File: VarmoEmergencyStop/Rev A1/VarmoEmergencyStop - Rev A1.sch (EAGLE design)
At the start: 6 parts, among them J1 22-05-7028-02, X1 NC3MAV, X2 NC3FAV2, X3 NC3MAV

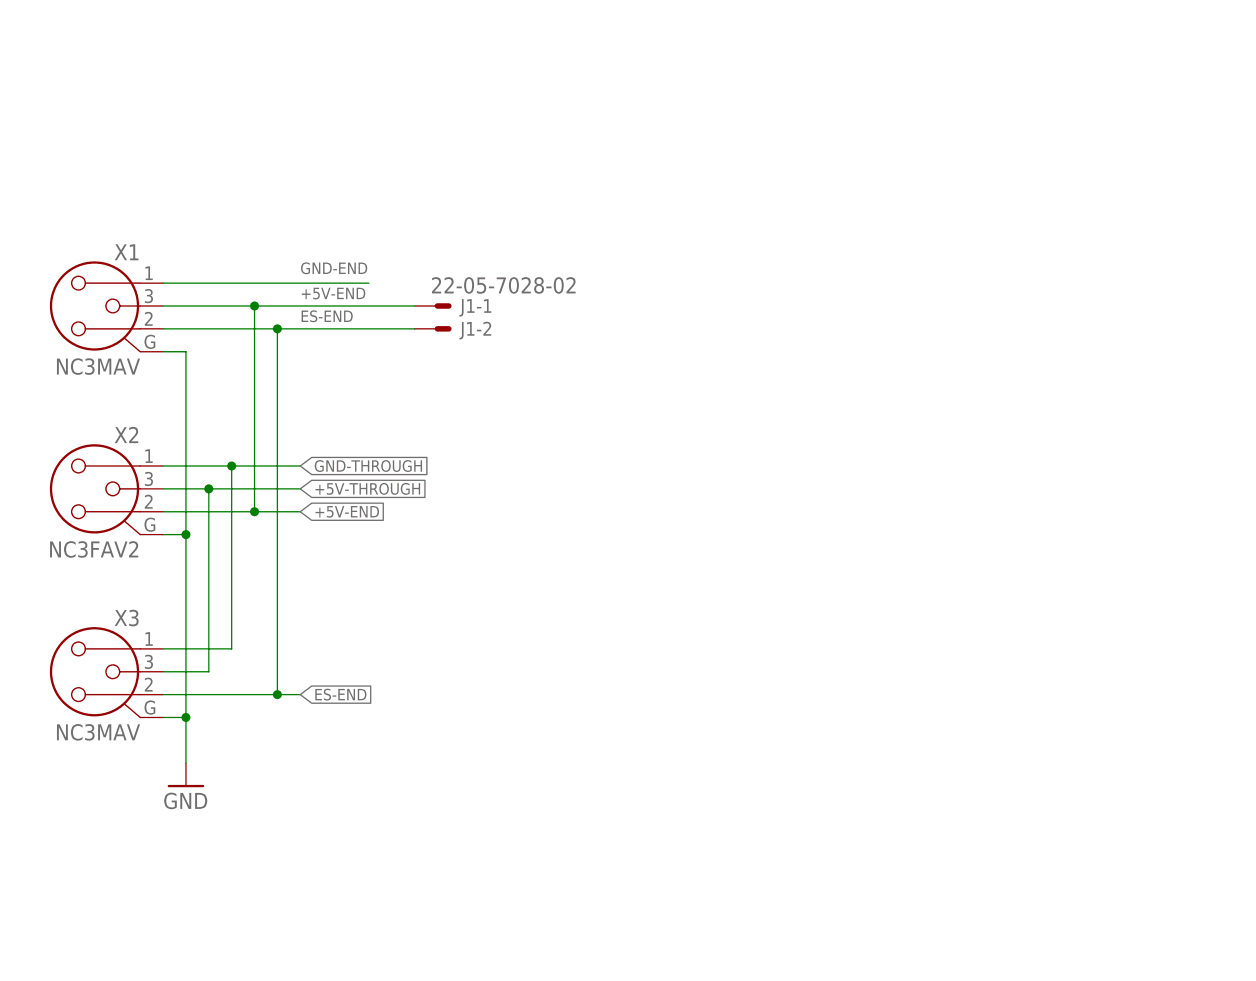
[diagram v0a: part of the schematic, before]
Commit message: Generate Gerber
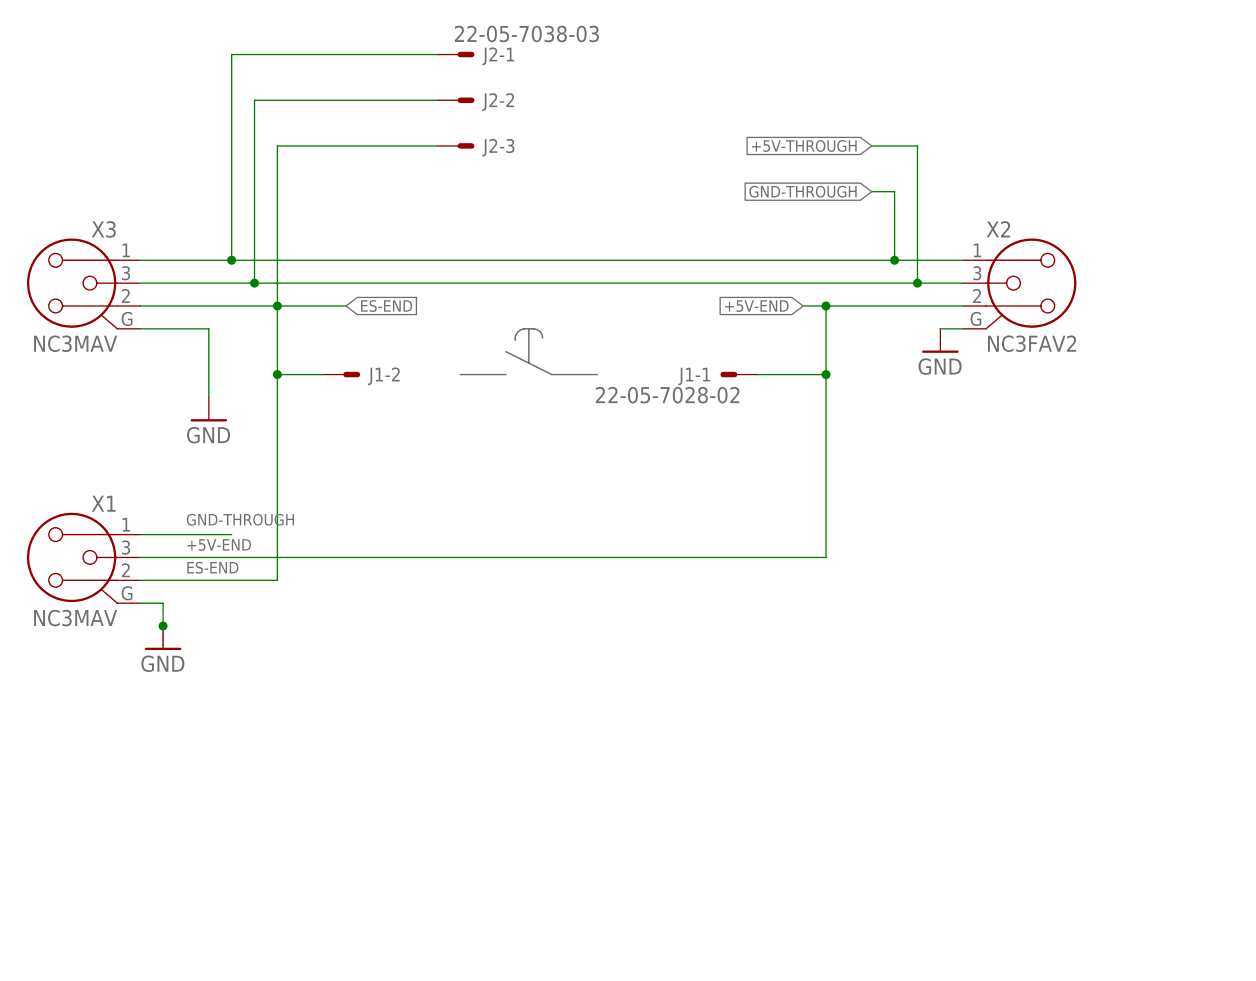
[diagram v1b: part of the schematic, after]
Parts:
- added J2: 22-05-7038-03, con-molex:22-05-7038-03
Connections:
- removed net GND-END: X1.1
- net +5V-THROUGH: now also J2-2.S
- net ES-END: now also J2-3.S
- net GND-THROUGH: now also J2-1.S, X1.1
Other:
- moved on the sheet: J1-1, J1-2, X1, X2, X3
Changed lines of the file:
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@@
 <part name="U$1" library="exmachina" deviceset="EXMACHINA-LOGO" device="-NAME"/>
 <part name="U$2" library="cc-by-sa" deviceset="CC-BY-NC-SA" device=""/>
+<part name="GND2" library="supply1" deviceset="GND" device=""/>
+<part name="GND3" library="supply1" deviceset="GND" device=""/>
+<part name="J2" library="con-molex" deviceset="22-?-03" device="05-7038"/>
 </parts>
 <sheets>
 <sheet>
 <plain>
+<wire x1="129.54" y1="142.24" x2="134.62" y2="142.24" width="0.1524" layer="97"/>
+<wire x1="139.7" y1="142.24" x2="144.78" y2="142.24" width="0.1524" layer="97"/>
+<wire x1="139.7" y1="142.24" x2="137.16" y2="143.51" width="0.1524" layer="97"/>
+<wire x1="137.16" y1="143.51" x2="134.62" y2="144.78" width="0.1524" layer="97"/>
+<wire x1="137.16" y1="143.51" x2="137.16" y2="147.32" width="0.1524" layer="97"/>
+<wire x1="136.652" y1="147.32" x2="137.668" y2="147.32" width="0.1524" layer="97"/>
+<wire x1="137.668" y1="147.32" x2="138.684" y2="146.304" width="0.1524" layer="97" curve="-90"/>
+<wire x1="136.652" y1="147.32" x2="135.636" y2="146.05" width="0.1524" layer="97" curve="90"/>
 </plain>
 <instances>
 <instance part="FRAME1" gate="G$1" x="0" y="0"/>
-<instance part="X1" gate="G$1" x="88.9" y="149.86" rot="MR0"/>
-<instance part="X3" gate="G$1" x="88.9" y="109.22" rot="MR0"/>
-<instance part="X2" gate="G$1" x="88.9" y="129.54" rot="MR0"/>
-<instance part="J1" gate="-1" x="127" y="149.86"/>
-<instance part="J1" gate="-2" x="127" y="147.32"/>
-<instance part="GND1" gate="1" x="99.06" y="96.52"/>
+<instance part="X1" gate="G$1" x="86.36" y="121.92" rot="MR0"/>
+<instance part="X3" gate="G$1" x="86.36" y="152.4" rot="MR0"/>
+<instance part="X2" gate="G$1" x="193.04" y="152.4"/>
+<instance part="J1" gate="-1" x="160.02" y="142.24" rot="R180"/>
+<instance part="J1" gate="-2" x="116.84" y="142.24"/>
+<instance part="GND1" gate="1" x="101.6" y="137.16"/>
 <instance part="U$1" gate="G$1" x="315.468" y="18.796"/>
 <instance part="U$2" gate="G$1" x="309.118" y="8.89"/>
+<instance part="GND2" gate="1" x="182.88" y="144.78"/>
+<instance part="GND3" gate="1" x="96.52" y="111.76"/>
+<instance part="J2" gate="-1" x="129.54" y="177.8"/>
+<instance part="J2" gate="-2" x="129.54" y="172.72"/>
+<instance part="J2" gate="-3" x="129.54" y="167.64"/>
 </instances>
 <busses>
@@
 <segment>
 <pinref part="X2" gate="G$1" pin="3"/>
-<wire x1="96.52" y1="129.54" x2="101.6" y2="129.54" width="0.1524" layer="91"/>
+<wire x1="185.42" y1="152.4" x2="180.34" y2="152.4" width="0.1524" layer="91"/>
 <pinref part="X3" gate="G$1" pin="3"/>
-<wire x1="101.6" y1="129.54" x2="111.76" y2="129.54" width="0.1524" layer="91"/>
-<wire x1="96.52" y1="109.22" x2="101.6" y2="109.22" width="0.1524" layer="91"/>
-<wire x1="101.6" y1="109.22" x2="101.6" y2="129.54" width="0.1524" layer="91"/>
-<junction x="101.6" y="129.54"/>
-<label x="111.76" y="129.54" size="1.27" layer="95" xref="yes"/>
+<wire x1="180.34" y1="152.4" x2="180.34" y2="167.64" width="0.1524" layer="91"/>
+<wire x1="180.34" y1="167.64" x2="175.26" y2="167.64" width="0.1524" layer="91"/>
+<wire x1="93.98" y1="152.4" x2="106.68" y2="152.4" width="0.1524" layer="91"/>
+<junction x="180.34" y="152.4"/>
+<label x="175.26" y="167.64" size="1.27" layer="95" rot="MR0" xref="yes"/>
+<pinref part="J2" gate="-2" pin="S"/>
+<wire x1="106.68" y1="152.4" x2="180.34" y2="152.4" width="0.1524" layer="91"/>
+<wire x1="106.68" y1="152.4" x2="106.68" y2="172.72" width="0.1524" layer="91"/>
+<wire x1="106.68" y1="172.72" x2="127" y2="172.72" width="0.1524" layer="91"/>
+<junction x="106.68" y="152.4"/>
 </segment>
 </net>
@@
 <segment>
 <pinref part="X1" gate="G$1" pin="G"/>
-<wire x1="96.52" y1="144.78" x2="99.06" y2="144.78" width="0.1524" layer="91"/>
-<wire x1="99.06" y1="144.78" x2="99.06" y2="124.46" width="0.1524" layer="91"/>
+<wire x1="93.98" y1="116.84" x2="96.52" y2="116.84" width="0.1524" layer="91"/>
+<wire x1="96.52" y1="114.3" x2="96.52" y2="116.84" width="0.1524" layer="91"/>
+<pinref part="GND3" gate="1" pin="GND"/>
+<junction x="96.52" y="114.3"/>
+</segment>
+<segment>
+<pinref part="X2" gate="G$1" pin="G"/>
+<wire x1="185.42" y1="147.32" x2="182.88" y2="147.32" width="0.1524" layer="91"/>
+<pinref part="GND2" gate="1" pin="GND"/>
+</segment>
+<segment>
 <pinref part="X3" gate="G$1" pin="G"/>
-<wire x1="99.06" y1="124.46" x2="99.06" y2="104.14" width="0.1524" layer="91"/>
-<wire x1="99.06" y1="104.14" x2="99.06" y2="99.06" width="0.1524" layer="91"/>
-<wire x1="96.52" y1="104.14" x2="99.06" y2="104.14" width="0.1524" layer="91"/>
-<junction x="99.06" y="104.14"/>
-<pinref part="X2" gate="G$1" pin="G"/>
-<wire x1="96.52" y1="124.46" x2="99.06" y2="124.46" width="0.1524" layer="91"/>
-<junction x="99.06" y="124.46"/>
+<wire x1="101.6" y1="147.32" x2="101.6" y2="139.7" width="0.1524" layer="91"/>
+<wire x1="93.98" y1="147.32" x2="101.6" y2="147.32" width="0.1524" layer="91"/>
 <pinref part="GND1" gate="1" pin="GND"/>
-</segment>
-</net>
-<net name="GND-END" class="1">
-<segment>
-<pinref part="X1" gate="G$1" pin="1"/>
-<label x="111.76" y="153.416" size="1.27" layer="95"/>
-<wire x1="96.52" y1="152.4" x2="119.38" y2="152.4" width="0.1524" layer="91"/>
 </segment>
 </net>
@@
 <segment>
 <pinref part="X1" gate="G$1" pin="2"/>
-<wire x1="96.52" y1="147.32" x2="109.22" y2="147.32" width="0.1524" layer="91"/>
-<label x="111.76" y="148.082" size="1.27" layer="95"/>
+<wire x1="93.98" y1="119.38" x2="109.22" y2="119.38" width="0.1524" layer="91"/>
+<wire x1="109.22" y1="119.38" x2="109.22" y2="142.24" width="0.1524" layer="91"/>
+<label x="99.06" y="120.142" size="1.27" layer="95"/>
 <pinref part="J1" gate="-2" pin="S"/>
 <pinref part="X3" gate="G$1" pin="2"/>
-<wire x1="109.22" y1="147.32" x2="124.46" y2="147.32" width="0.1524" layer="91"/>
-<wire x1="96.52" y1="106.68" x2="109.22" y2="106.68" width="0.1524" layer="91"/>
-<label x="111.76" y="106.68" size="1.27" layer="95" xref="yes"/>
-<wire x1="109.22" y1="106.68" x2="111.76" y2="106.68" width="0.1524" layer="91"/>
-<wire x1="109.22" y1="147.32" x2="109.22" y2="106.68" width="0.1524" layer="91"/>
-<junction x="109.22" y="147.32"/>
-<junction x="109.22" y="106.68"/>
+<wire x1="109.22" y1="142.24" x2="114.3" y2="142.24" width="0.1524" layer="91"/>
+<wire x1="93.98" y1="149.86" x2="109.22" y2="149.86" width="0.1524" layer="91"/>
+<label x="116.84" y="149.86" size="1.27" layer="95" xref="yes"/>
+<wire x1="109.22" y1="149.86" x2="116.84" y2="149.86" width="0.1524" layer="91"/>
+<junction x="109.22" y="142.24"/>
+<junction x="109.22" y="149.86"/>
+<wire x1="109.22" y1="142.24" x2="109.22" y2="149.86" width="0.1524" layer="91"/>
+<pinref part="J2" gate="-3" pin="S"/>
+<wire x1="109.22" y1="149.86" x2="109.22" y2="167.64" width="0.1524" layer="91"/>
+<wire x1="109.22" y1="167.64" x2="127" y2="167.64" width="0.1524" layer="91"/>
 </segment>
 </net>
@@
 <segment>
 <pinref part="X2" gate="G$1" pin="1"/>
-<wire x1="96.52" y1="132.08" x2="104.14" y2="132.08" width="0.1524" layer="91"/>
+<wire x1="185.42" y1="154.94" x2="177.8" y2="154.94" width="0.1524" layer="91"/>
 <pinref part="X3" gate="G$1" pin="1"/>
-<wire x1="96.52" y1="111.76" x2="104.14" y2="111.76" width="0.1524" layer="91"/>
-<wire x1="104.14" y1="132.08" x2="104.14" y2="111.76" width="0.1524" layer="91"/>
-<wire x1="104.14" y1="132.08" x2="111.76" y2="132.08" width="0.1524" layer="91"/>
-<junction x="104.14" y="132.08"/>
-<label x="111.76" y="132.08" size="1.27" layer="95" xref="yes"/>
+<wire x1="93.98" y1="154.94" x2="104.14" y2="154.94" width="0.1524" layer="91"/>
+<wire x1="104.14" y1="154.94" x2="177.8" y2="154.94" width="0.1524" layer="91"/>
+<wire x1="177.8" y1="154.94" x2="177.8" y2="162.56" width="0.1524" layer="91"/>
+<wire x1="177.8" y1="162.56" x2="175.26" y2="162.56" width="0.1524" layer="91"/>
+<junction x="177.8" y="154.94"/>
+<label x="175.26" y="162.56" size="1.27" layer="95" rot="MR0" xref="yes"/>
+<pinref part="J2" gate="-1" pin="S"/>
+<wire x1="104.14" y1="154.94" x2="104.14" y2="177.8" width="0.1524" layer="91"/>
+<wire x1="104.14" y1="177.8" x2="127" y2="177.8" width="0.1524" layer="91"/>
+<junction x="104.14" y="154.94"/>
+</segment>
+<segment>
+<pinref part="X1" gate="G$1" pin="1"/>
+<label x="99.06" y="125.476" size="1.27" layer="95"/>
+<wire x1="93.98" y1="124.46" x2="104.14" y2="124.46" width="0.1524" layer="91"/>
 </segment>
 </net>
@@
 <segment>
 <pinref part="X2" gate="G$1" pin="2"/>
-<wire x1="96.52" y1="127" x2="106.68" y2="127" width="0.1524" layer="91"/>
-<label x="111.76" y="127" size="1.27" layer="95" xref="yes"/>
+<wire x1="185.42" y1="149.86" x2="170.18" y2="149.86" width="0.1524" layer="91"/>
+<label x="167.64" y="149.86" size="1.27" layer="95" rot="MR0" xref="yes"/>
 <pinref part="X1" gate="G$1" pin="3"/>
-<label x="111.76" y="150.622" size="1.27" layer="95"/>
+<label x="99.06" y="122.682" size="1.27" layer="95"/>
 <pinref part="J1" gate="-1" pin="S"/>
-<wire x1="106.68" y1="127" x2="111.76" y2="127" width="0.1524" layer="91"/>
-<wire x1="124.46" y1="149.86" x2="106.68" y2="149.86" width="0.1524" layer="91"/>
-<wire x1="106.68" y1="149.86" x2="96.52" y2="149.86" width="0.1524" layer="91"/>
-<wire x1="106.68" y1="127" x2="106.68" y2="149.86" width="0.1524" layer="91"/>
-<junction x="106.68" y="127"/>
-<junction x="106.68" y="149.86"/>
+<wire x1="170.18" y1="149.86" x2="167.64" y2="149.86" width="0.1524" layer="91"/>
+<wire x1="162.56" y1="142.24" x2="170.18" y2="142.24" width="0.1524" layer="91"/>
+<wire x1="170.18" y1="121.92" x2="93.98" y2="121.92" width="0.1524" layer="91"/>
+<wire x1="170.18" y1="149.86" x2="170.18" y2="142.24" width="0.1524" layer="91"/>
+<wire x1="170.18" y1="121.92" x2="170.18" y2="142.24" width="0.1524" layer="91"/>
+<junction x="170.18" y="149.86"/>
+<junction x="170.18" y="142.24"/>
 </segment>
 </net>
